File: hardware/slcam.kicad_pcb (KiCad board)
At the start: 2 copper layers, 2 parts, among them U1 STM32F103C8Tx, Y1 Crystal

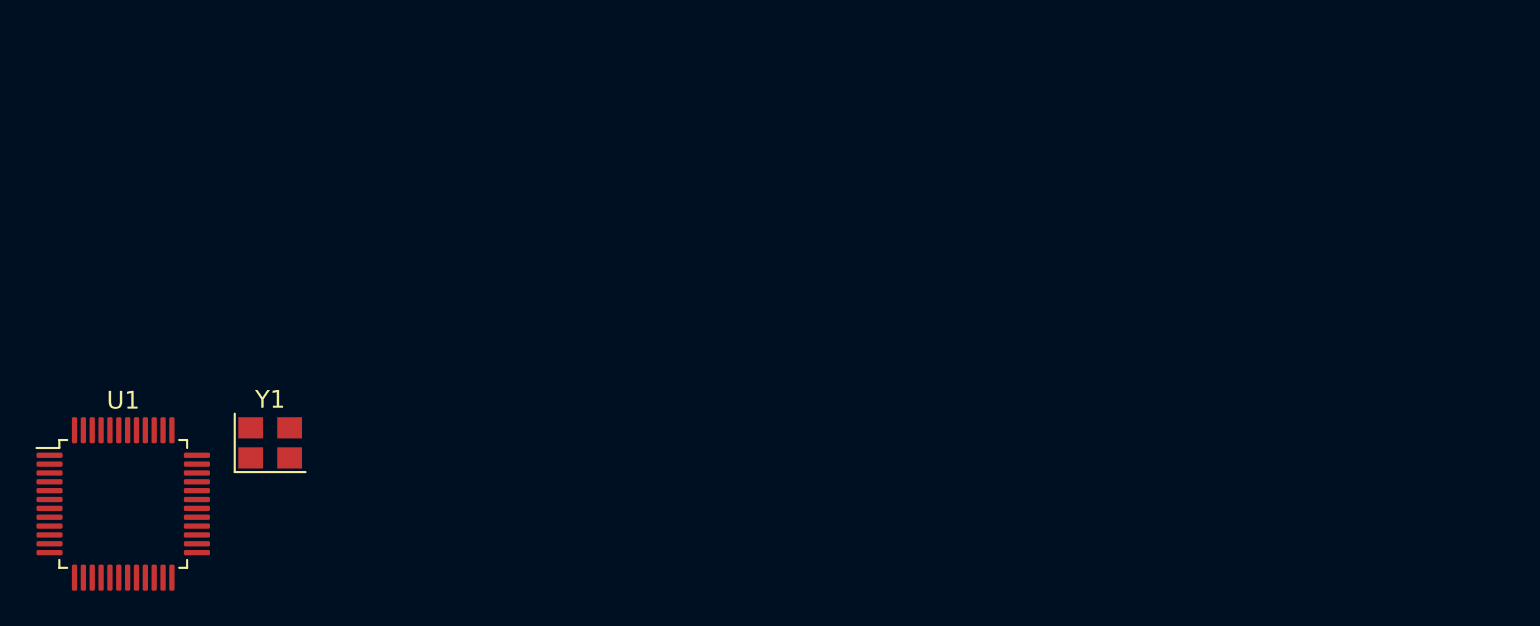
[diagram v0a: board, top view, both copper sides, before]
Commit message: Initial layout
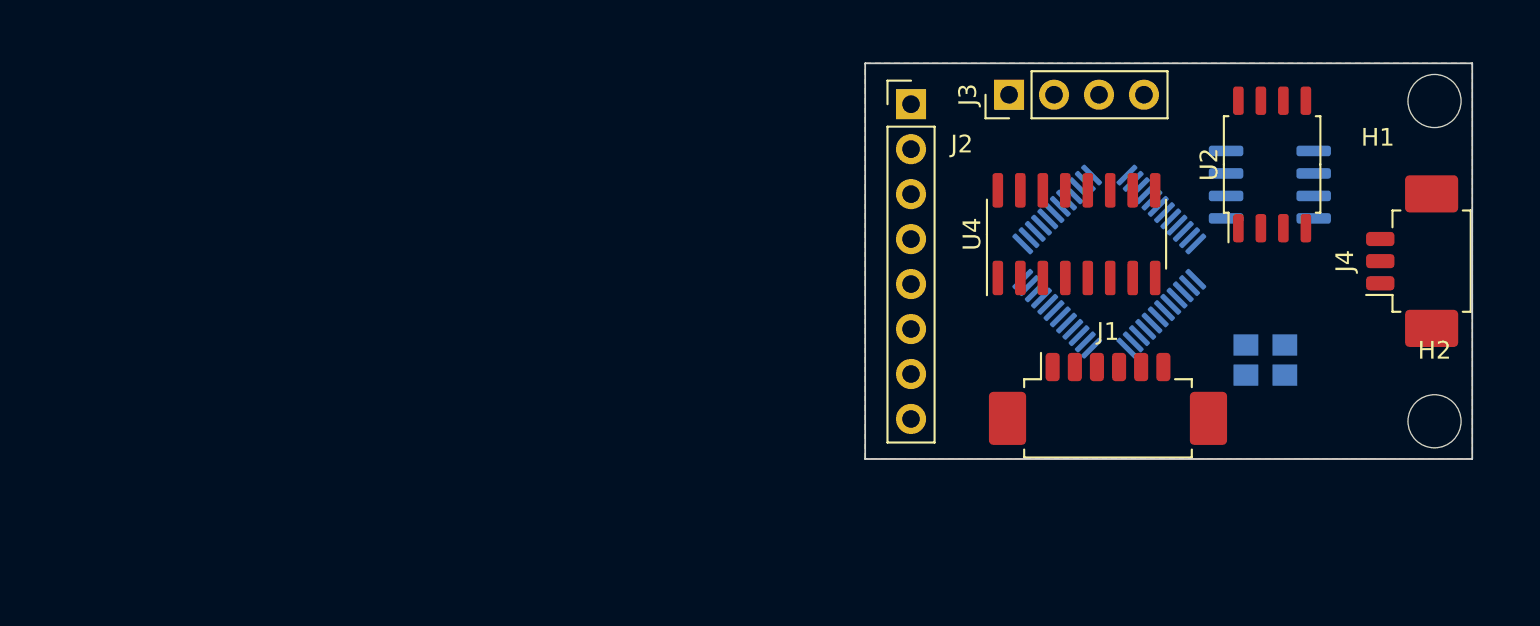
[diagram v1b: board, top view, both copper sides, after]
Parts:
- added H1: MountingHole, MountingHole:MountingHole_3mm, F.Cu at (235.4, 53.4)
- added H2: MountingHole, MountingHole:MountingHole_3mm, F.Cu at (235.4, 71.5)
- added J1: 532610671, Connector_Molex:Molex_PicoBlade_53261-0671_1x06-1MP_P1.25mm_Horizontal, F.Cu at (216.9, 70.9)
- added J2: Conn_01x08, Connector_PinHeader_2.54mm:PinHeader_1x08_P2.54mm_Vertical, F.Cu at (205.8, 53.6)
- added J3: Conn_01x04, Connector_PinHeader_2.54mm:PinHeader_1x04_P2.54mm_Vertical, F.Cu at (211.3, 53.1)
- added J4: 532610371, Connector_Molex:Molex_PicoBlade_53261-0371_1x03-1MP_P1.25mm_Horizontal, F.Cu at (234.7, 62.5)
- added U2: W25Q128JVS, Package_SO:SOIC-8_5.23x5.23mm_P1.27mm, F.Cu at (226.2, 57.0)
- added U3: TCAN330G, Package_SO:SOIC-8_3.9x4.9mm_P1.27mm, B.Cu at (226.1, 58.2)
- added U4: TPS2044D, Package_SO:SOIC-16_3.9x9.9mm_P1.27mm, F.Cu at (215.1, 61.0)
- U1: moved to B.Cu
- Y1: value Crystal -> Crystal_GND24; moved to B.Cu
- moved U1 57.4 mm to (217.0, 62.5), turned to 315 degrees
- moved Y1 56.4 mm to (225.8, 68.1)
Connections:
- Y1 pad 3: (no net) -> Net-(Y1-Pad3)
- Y1 pad 4: (no net) -> Net-(Y1-Pad4)
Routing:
- added copper zone on B.Cu, net (none)
- added copper zone on F.Cu, net (none)
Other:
- board outline added: 34.3 x 22.3 mm

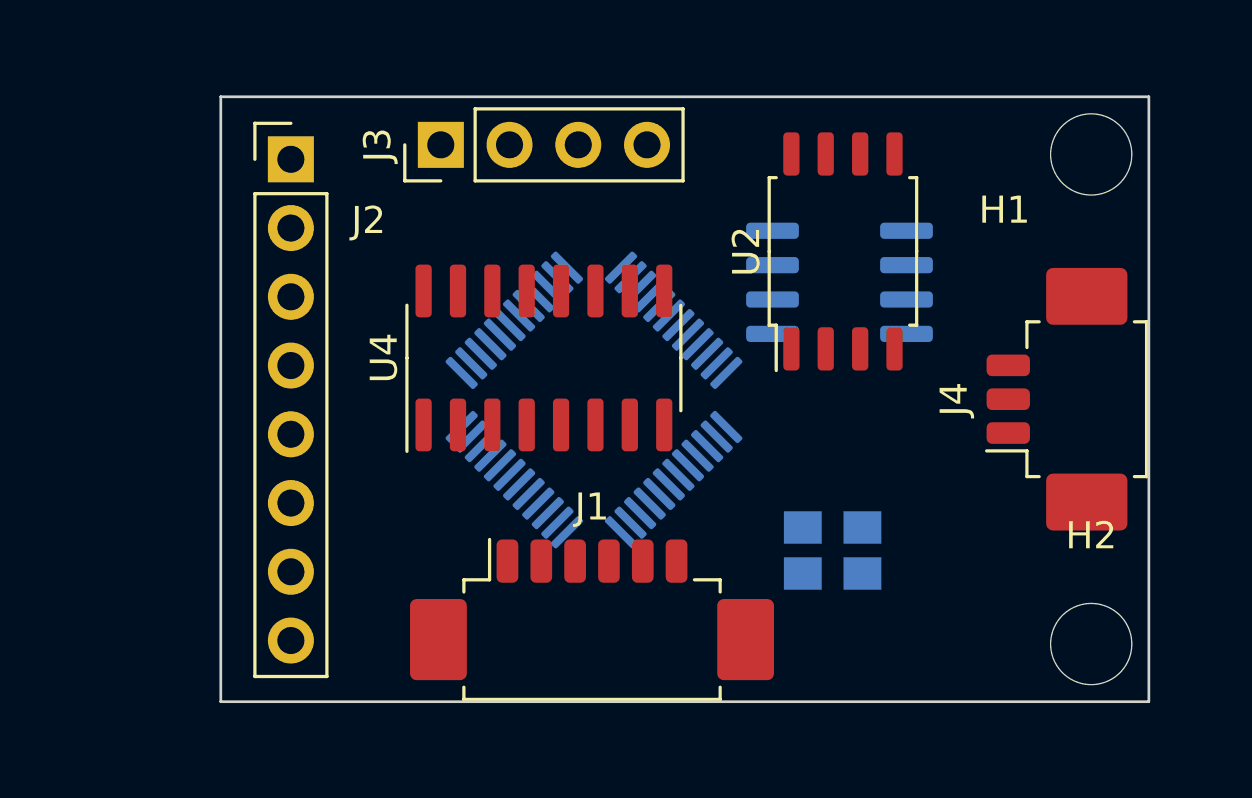
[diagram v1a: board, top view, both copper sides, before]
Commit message: General fixes #8 #9
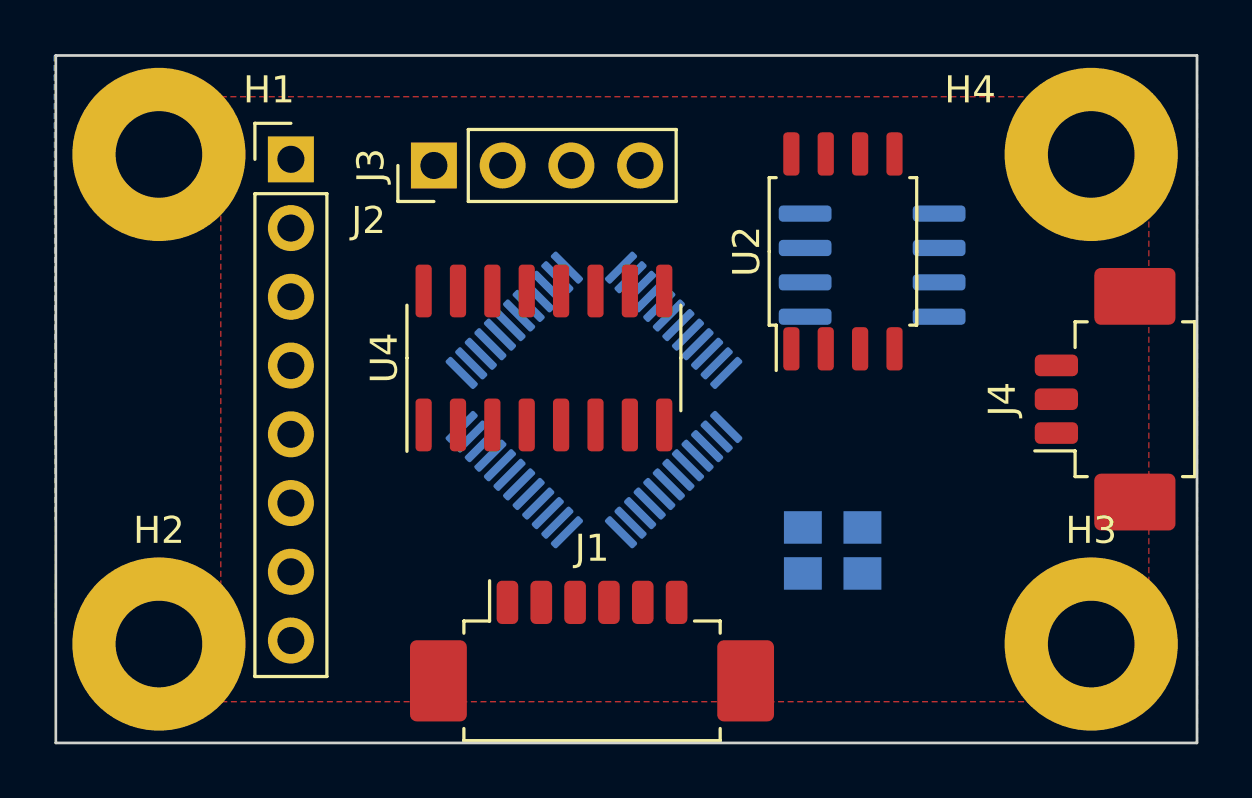
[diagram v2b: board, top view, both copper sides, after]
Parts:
- added H3: MountingHole, MountingHole:MountingHole_3.2mm_M3_Pad, F.Cu at (235.4, 71.5)
- added H4: MountingHole, MountingHole:MountingHole_3.2mm_M3_Pad, F.Cu at (235.4, 53.4)
- H1, H2: footprint MountingHole:MountingHole_3mm -> MountingHole:MountingHole_3.2mm_M3_Pad
- moved H1 34.4 mm to (200.9, 53.4)
- moved H2 34.4 mm to (200.9, 71.5)
- moved J4 1.78 mm to (236.5, 62.5)
- moved J1 1.52 mm to (216.9, 72.4)
- moved U3 1.36 mm to (227.3, 57.5)
- moved J3 0.80 mm to (211.1, 53.8)
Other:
- board size 34.3 x 22.3 mm -> 42.2 x 25.4 mm
